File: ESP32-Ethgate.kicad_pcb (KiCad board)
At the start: 2 copper layers, 76.2 x 38.1 mm, 54 parts, among them J1 USB_B_Micro, J2 HR911105A, Q1 UMH3N, U1 HT7233, U2 ESP32-WROOM-32U, U3 CH340C, U4 HT7233, U5 LAN8720A, U6 USBLC6-2SC6

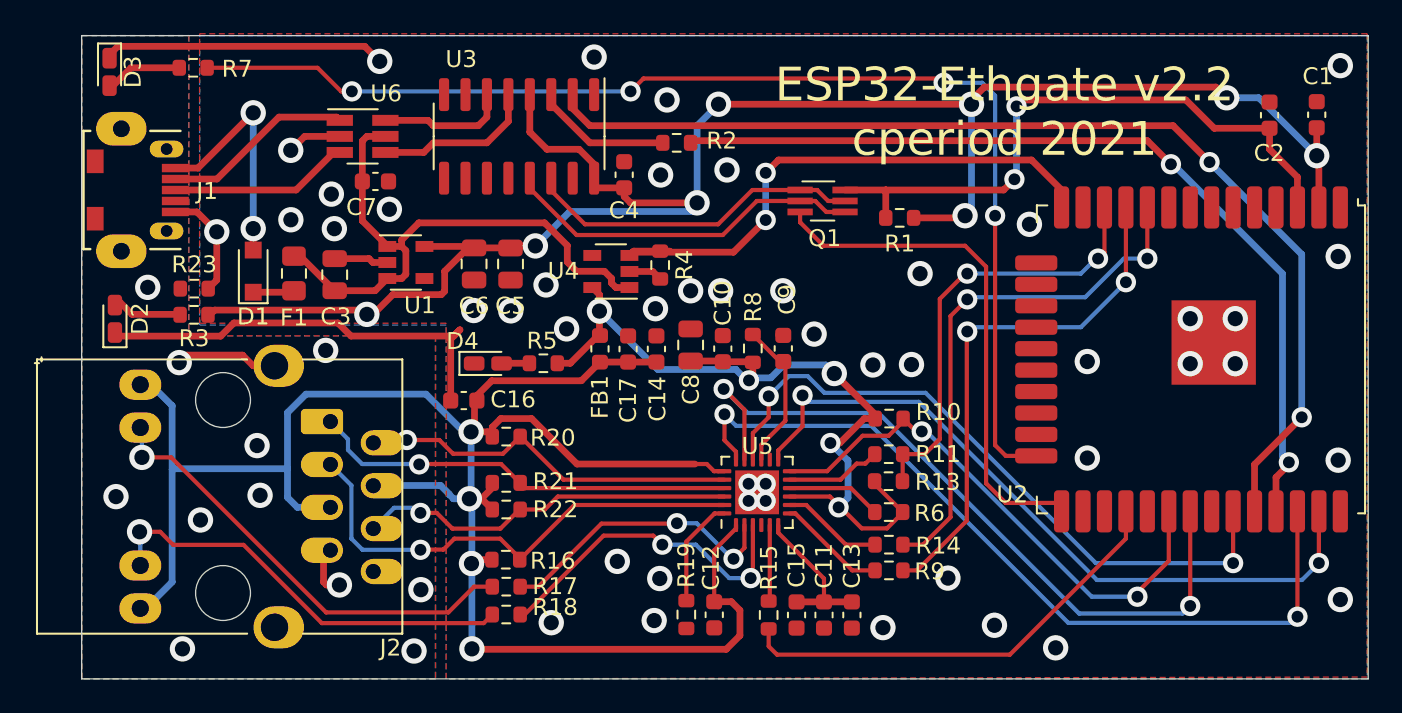
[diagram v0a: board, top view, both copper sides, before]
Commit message: more layout tweaks
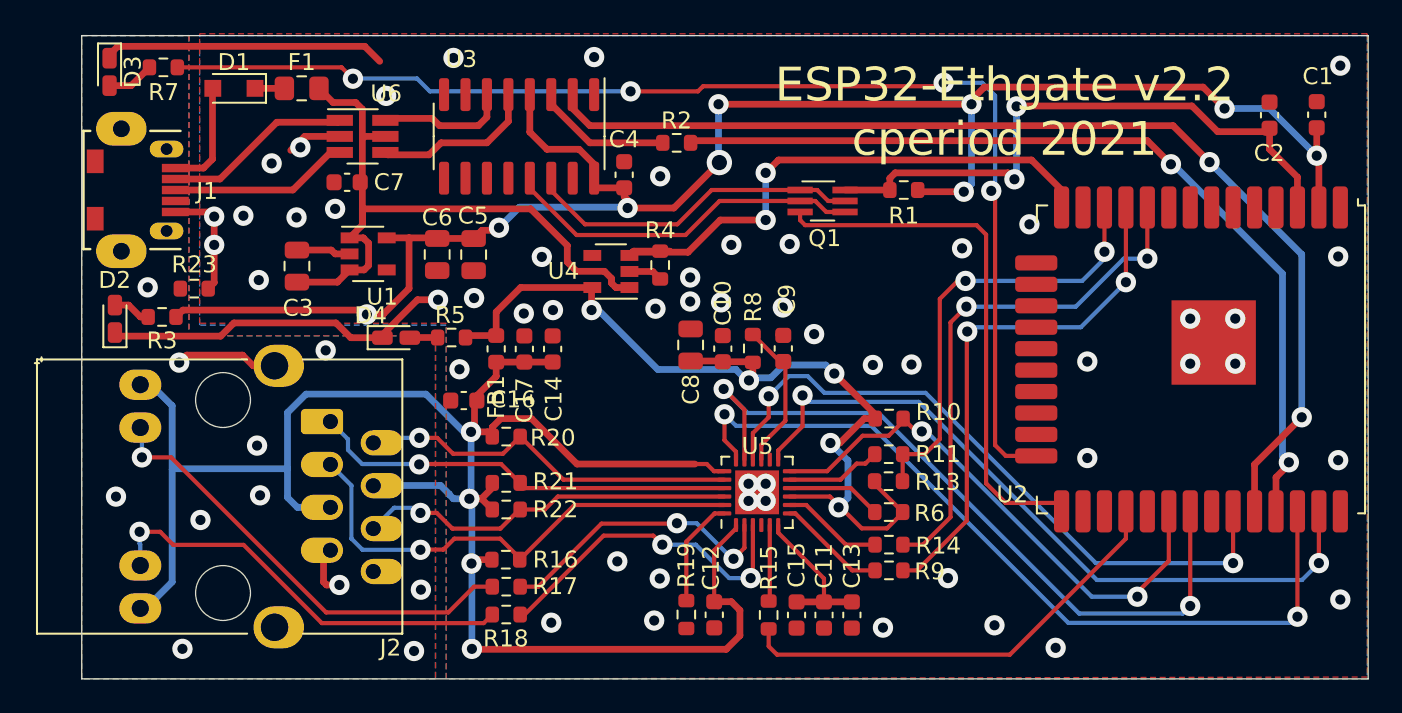
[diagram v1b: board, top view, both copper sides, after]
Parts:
- moved F1 11.0 mm to (80.3, 64.1), turned to 180 degrees
- moved D1 10.9 mm to (76.3, 64.1), turned to 180 degrees
- moved C14 6.15 mm to (95.2, 79.5)
- moved C17 6.15 mm to (93.5, 79.5)
- moved FB1 6.15 mm to (91.9, 79.5)
- moved D4 5.65 mm to (85.9, 78.9)
- moved R5 5.65 mm to (89.2, 78.8)
- moved U1 2.29 mm to (84.3, 73.9)
- moved C3 2.29 mm to (80.1, 74.6)
- moved C5 2.25 mm to (90.5, 73.9)
- moved C6 2.25 mm to (88.4, 73.9)
- moved R3 1.90 mm to (72.1, 77.6)
- moved R7 1.76 mm to (72.1, 62.8)
- moved C7 1.68 mm to (83.0, 69.6), turned to 180 degrees
- moved R1 1.67 mm to (116.0, 70.1)
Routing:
- net Net-(D1-Pad2): track 14.1 -> 6.62 mm, vias 2 -> 0
- net +3.3VA: track 121.2 -> 115.6 mm
- net /+3V3_LAN: track 49.5 -> 54.8 mm
- net GND: track 57.2 -> 52.8 mm, vias 46 -> 52
- net +3V3: track 110.1 -> 106.0 mm, vias 8 -> 9
- net +5V: track 35.7 -> 39.1 mm
- net Net-(D2-Pad2): track 4.32 -> 2.26 mm
- net Net-(D3-Pad2): track 4.65 -> 2.81 mm
- net /SLED: track 71.9 -> 73.7 mm
- net /EN: track 38.0 -> 37.0 mm
- net /IO0: track 30.5 -> 31.5 mm
- net Net-(D1-Pad1): track 2.45 -> 1.92 mm
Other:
- net class Default: via_drill 0.7 -> 0.6
- rule via_min_drill: 0.7 -> 0.6
